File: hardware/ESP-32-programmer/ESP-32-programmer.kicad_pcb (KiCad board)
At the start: 2 copper layers, 100 x 45 mm, 17 parts, among them J1 GS2, J2 CONN_01X06, J3 CONN_02X10, J4 CONN_02X10, J5 CONN_02X10, J6 CONN_01X06, J7 GS2, SW1 SW_DIP_x02, SW2 SW_Push, U1 LD1117S33TR_SOT223, U2 ESP-32-module

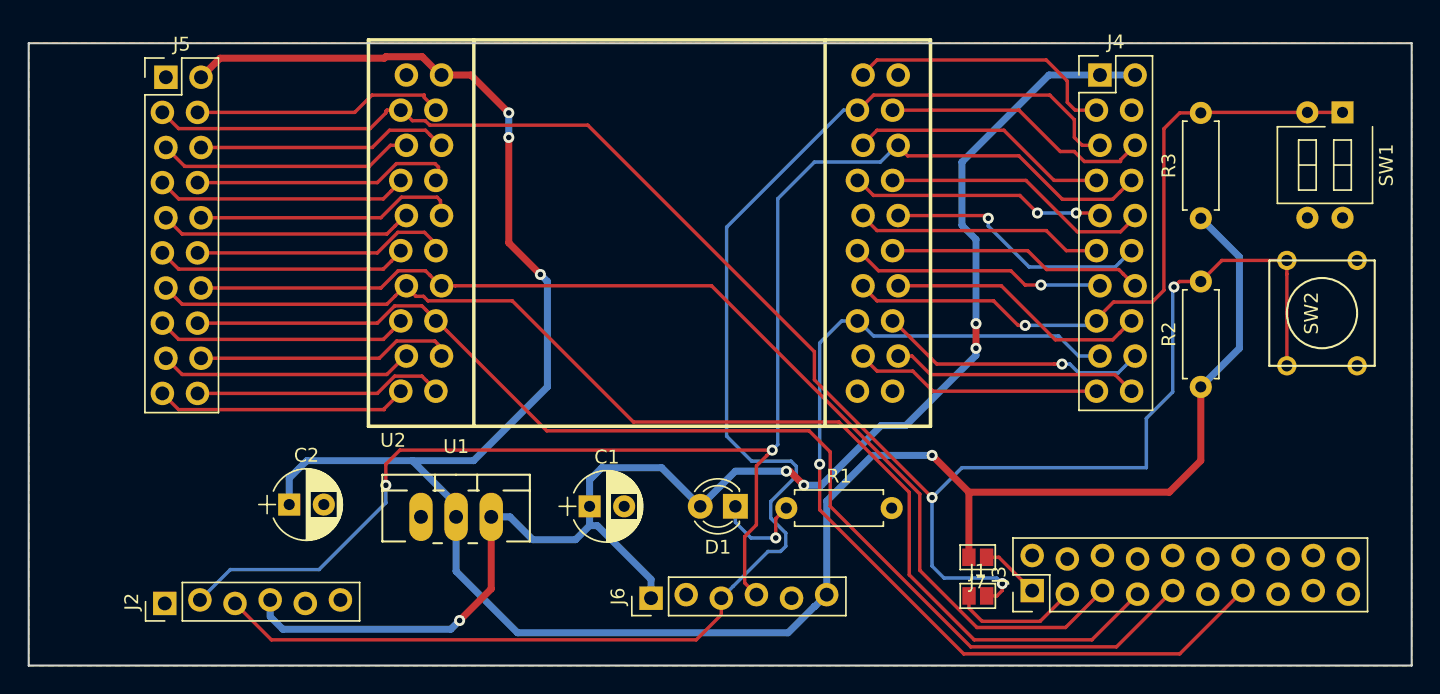
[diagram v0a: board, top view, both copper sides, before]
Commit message: Change module in ESP32 programmer
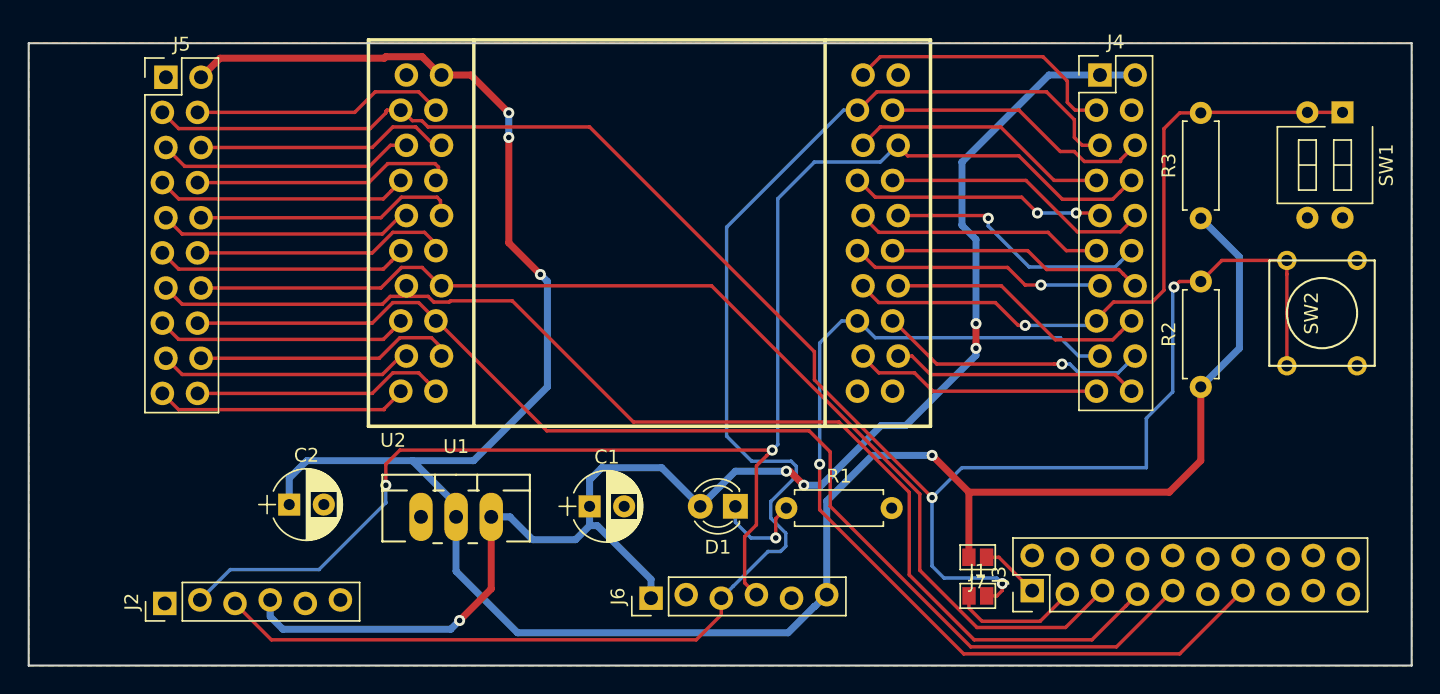
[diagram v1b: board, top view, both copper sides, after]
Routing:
- net /TMS: track 86.8 -> 86.2 mm
